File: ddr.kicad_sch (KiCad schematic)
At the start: 32 parts, among them U2 K4B4G1646Q, U3 K4B4G1646Q

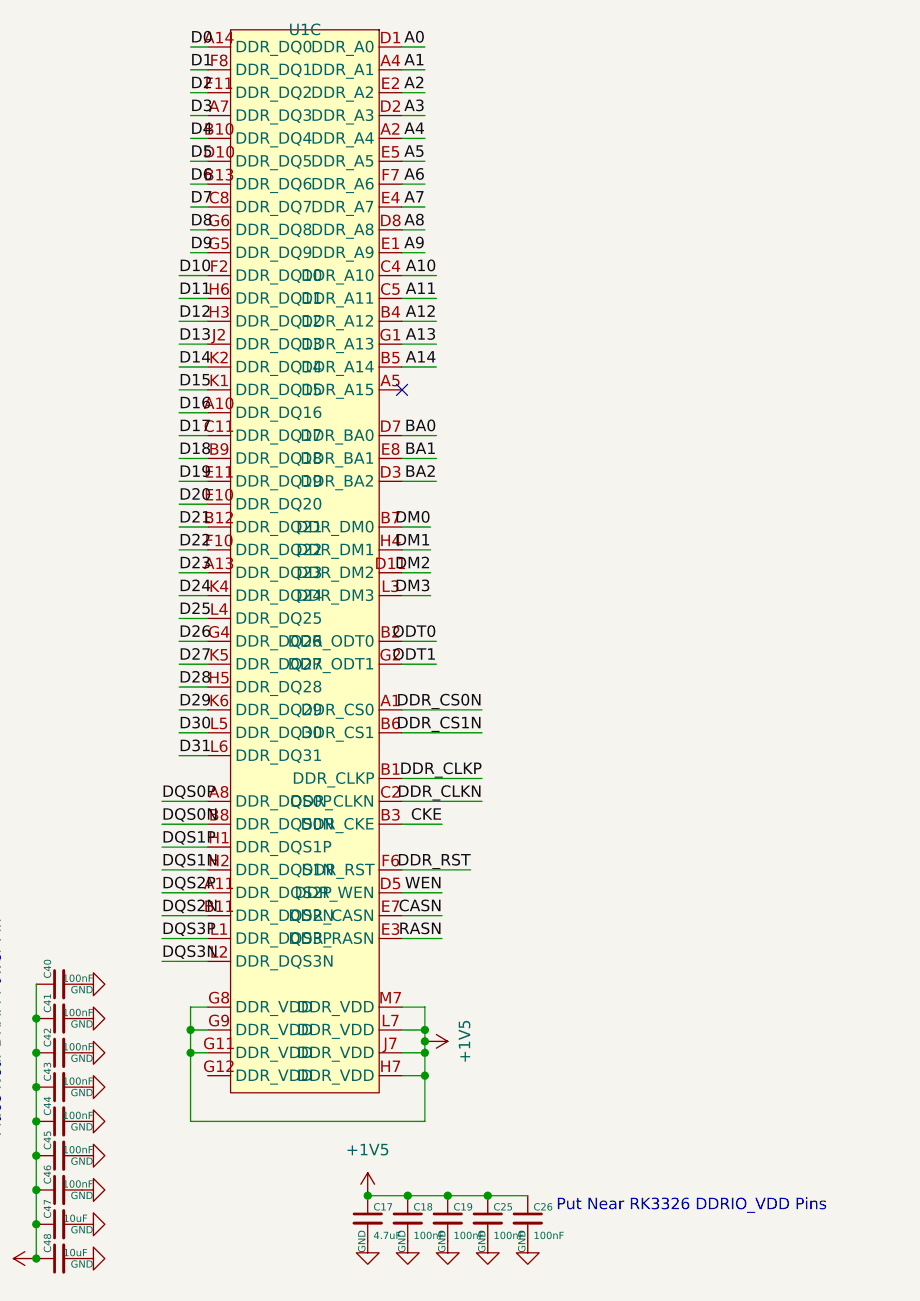
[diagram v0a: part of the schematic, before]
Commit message: file sync
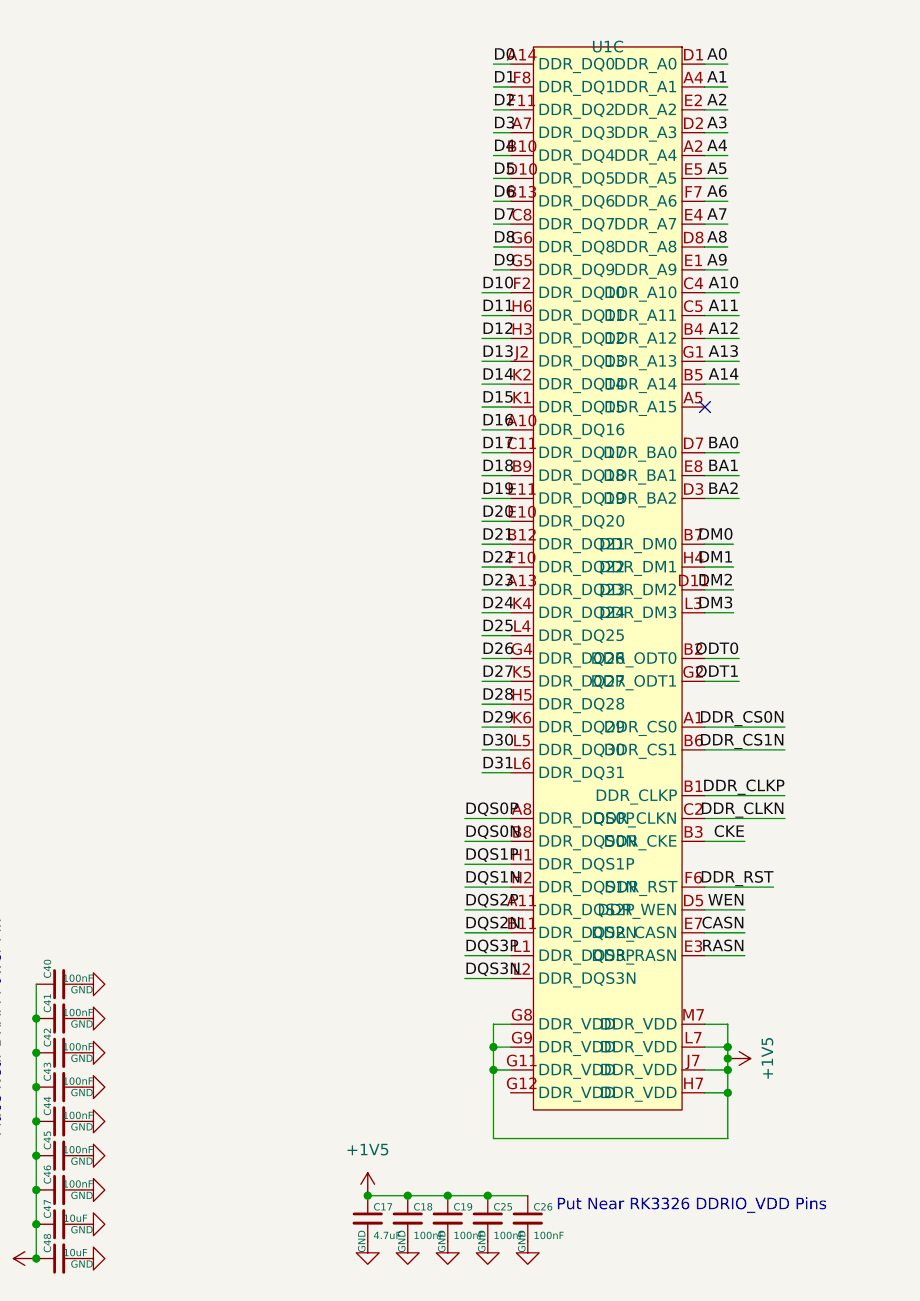
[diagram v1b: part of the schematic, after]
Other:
- moved on the sheet: U1C
